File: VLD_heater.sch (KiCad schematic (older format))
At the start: 10 parts

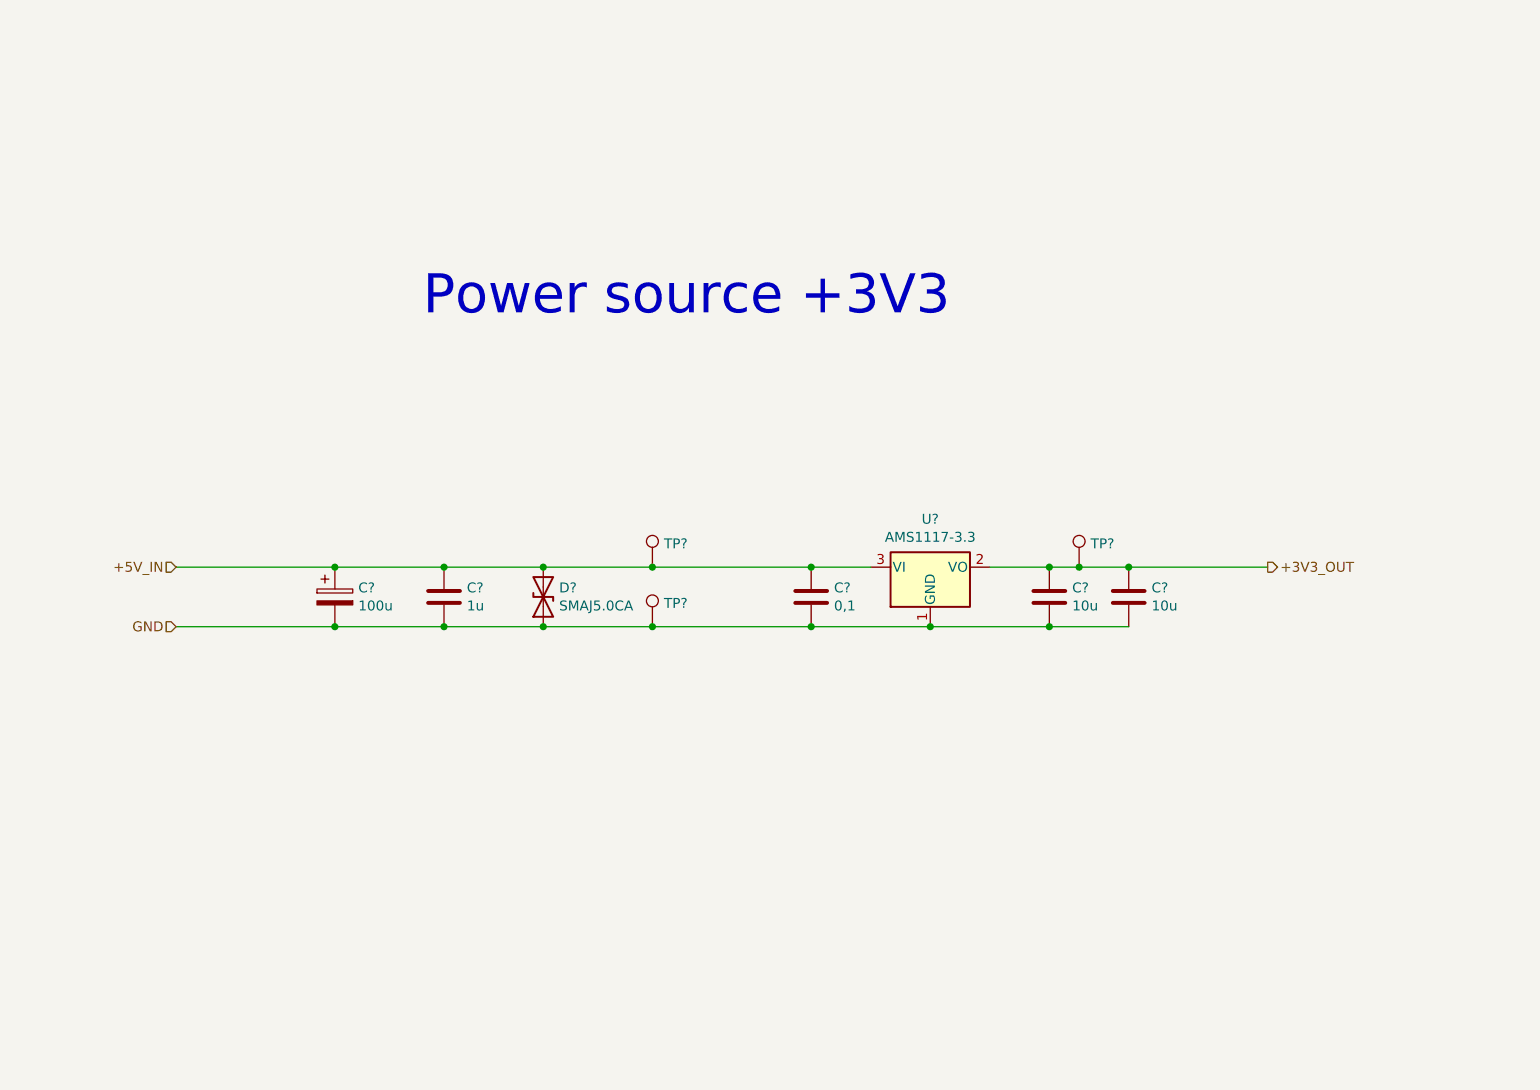
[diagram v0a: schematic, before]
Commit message: Add files via upload
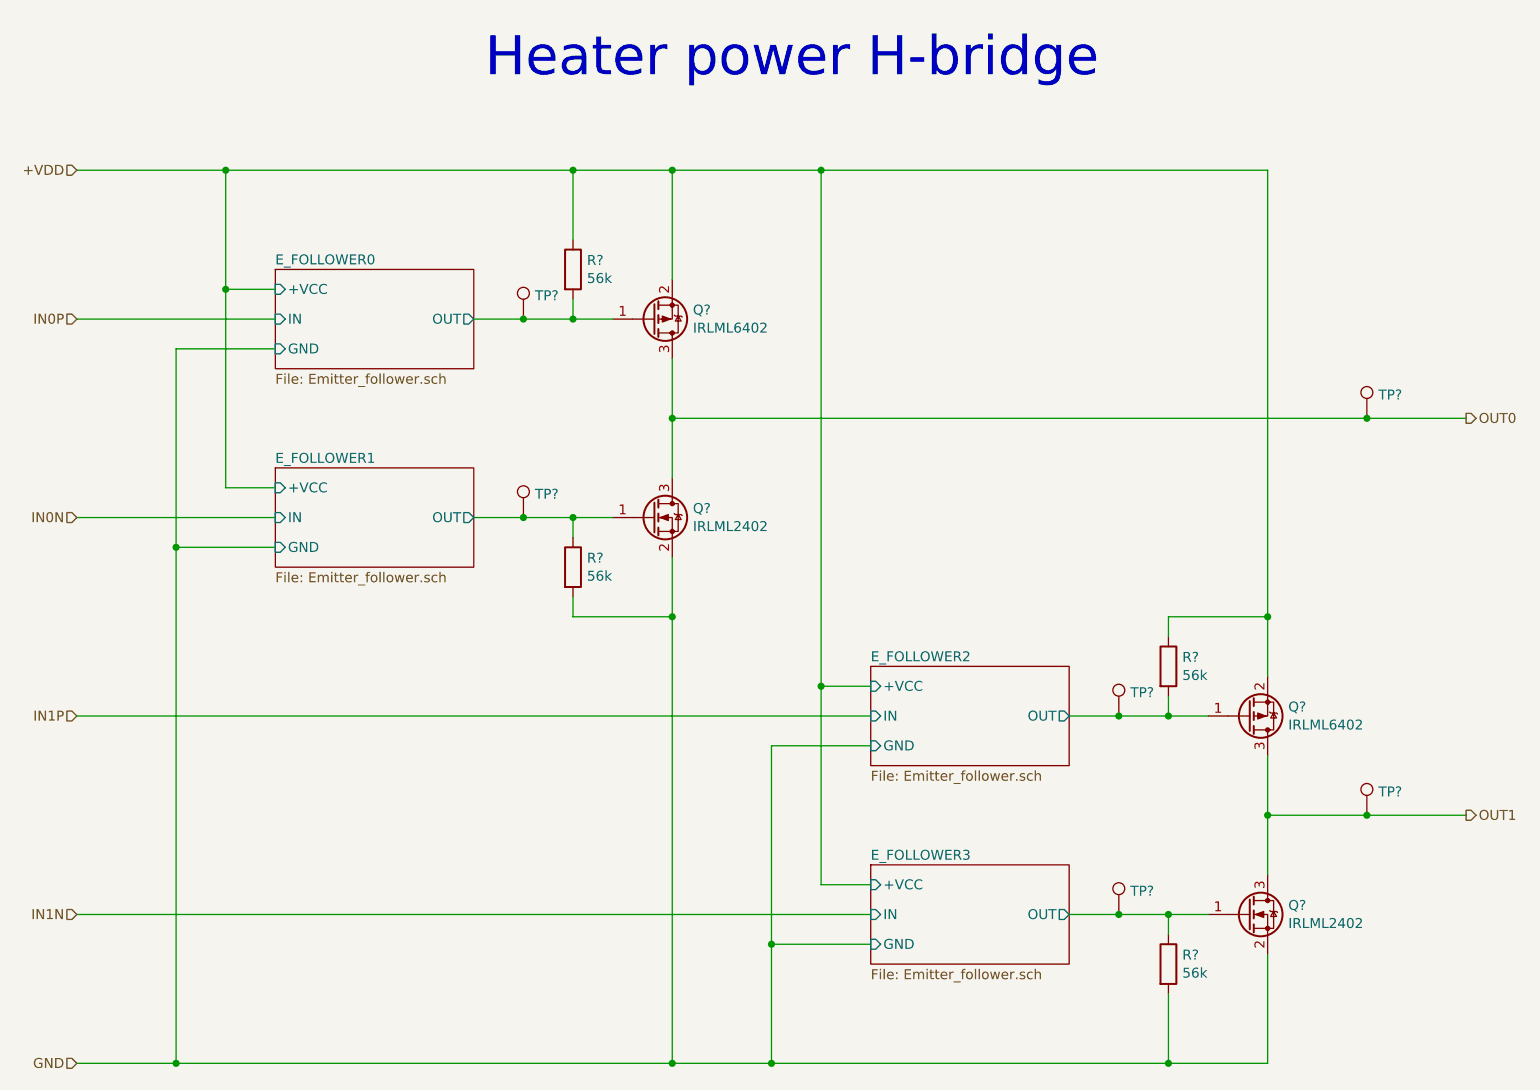
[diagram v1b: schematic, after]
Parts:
- removed C? (x2): 10u, Capacitor_SMD:C_1206_3216Metric_Pad1.33x1.80mm_HandSolder, symbol Device:C
- removed C?: 100u, symbol Device:CP
- removed C?: 0,1, Capacitor_SMD:C_0603_1608Metric_Pad1.08x0.95mm_HandSolder, symbol Device:C
- removed C?: 1u, Capacitor_SMD:C_0603_1608Metric_Pad1.08x0.95mm_HandSolder, symbol Device:C
- removed D?: SMAJ5.0CA, symbol Device:D_TVS
- removed TP? (x3): TestPoint, symbol Connector:TestPoint
- removed U?: AMS1117-3.3, Package_TO_SOT_SMD:SOT-223-3_TabPin2, symbol Regulator_Linear:AMS1117-3.3
- added Q? (x2): IRLML6402, Package_TO_SOT_SMD:SOT-23, symbol Transistor_FET:IRLML6402
- added Q? (x2): IRLML2402, Package_TO_SOT_SMD:SOT-23, symbol Transistor_FET:IRLML2060
- added R? (x4): 56k, Resistor_SMD:R_0603_1608Metric_Pad0.98x0.95mm_HandSolder, symbol Device:R
- added TP? (x6): TestPoint, symbol Connector:TestPoint
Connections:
- net GND: now also Q?.2 (S), Q?.2 (S), R?.2, R?.2
- new net +VDD: Q?.2 (S), Q?.2 (S), R?.1, R?.1
- new net E_FOLLOWER0/OUT: Q?.1 (G), R?.2, TP?.1
- new net E_FOLLOWER1/OUT: Q?.1 (G), R?.1, TP?.1
- new net E_FOLLOWER2/OUT: Q?.1 (G), R?.2, TP?.1
- new net E_FOLLOWER3/OUT: Q?.1 (G), R?.1, TP?.1
- new net OUT0: Q?.3 (D), Q?.3 (D), TP?.1
- new net OUT1: Q?.3 (D), Q?.3 (D), TP?.1
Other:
- note added: "Heater power H-bridge"
- note removed: "Power source +3V3"
